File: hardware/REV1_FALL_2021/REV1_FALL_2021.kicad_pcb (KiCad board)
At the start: 2 copper layers, 146 x 133.4 mm, 34 parts, among them J101 Screw_Terminal_01x02, Q101 Q_NMOS_GDS, U1 Teensy3.6_All_Pins, U2 PA16165_Breakout, U201 TPS2113ADRBR, U3 MPL3115A2_Breakout, U301 TPS2113ADRBR, U4 BNO055_Breakout, U5 RFM69HCW_Breakout

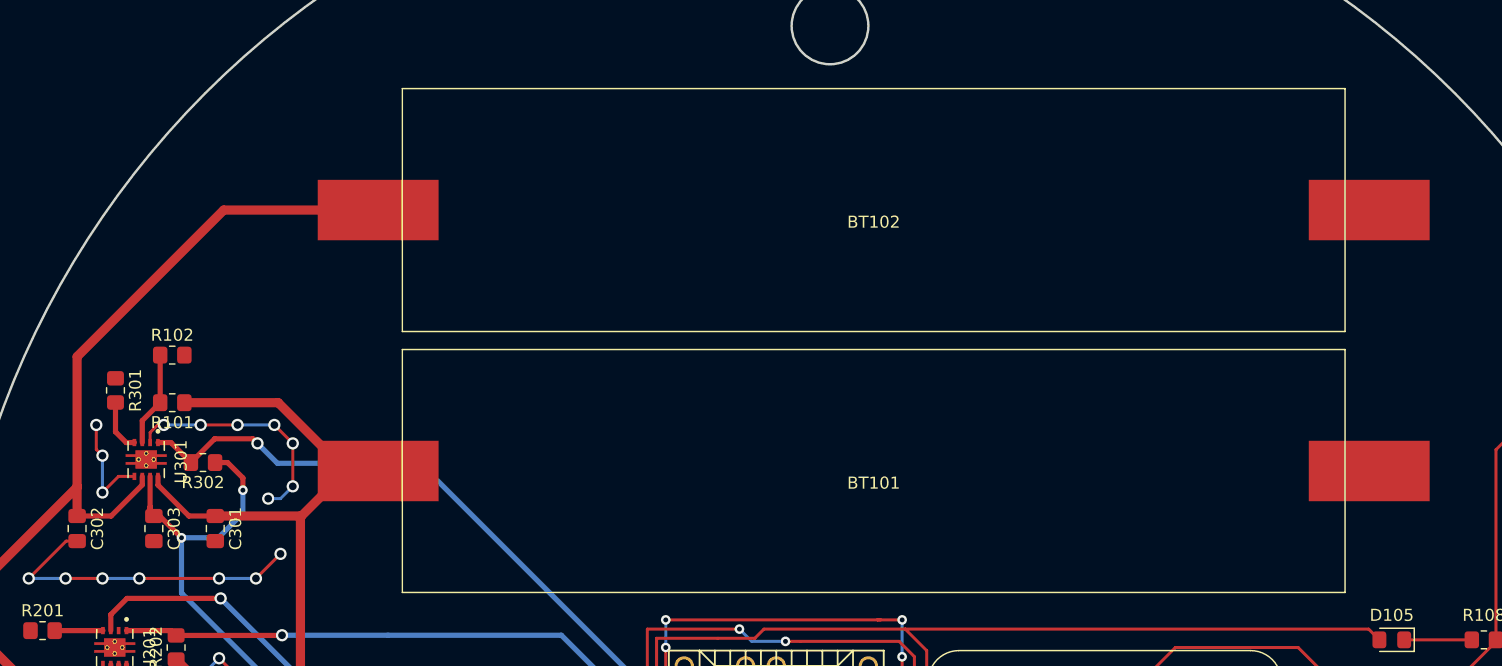
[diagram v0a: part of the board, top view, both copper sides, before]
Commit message: tweak battery positions
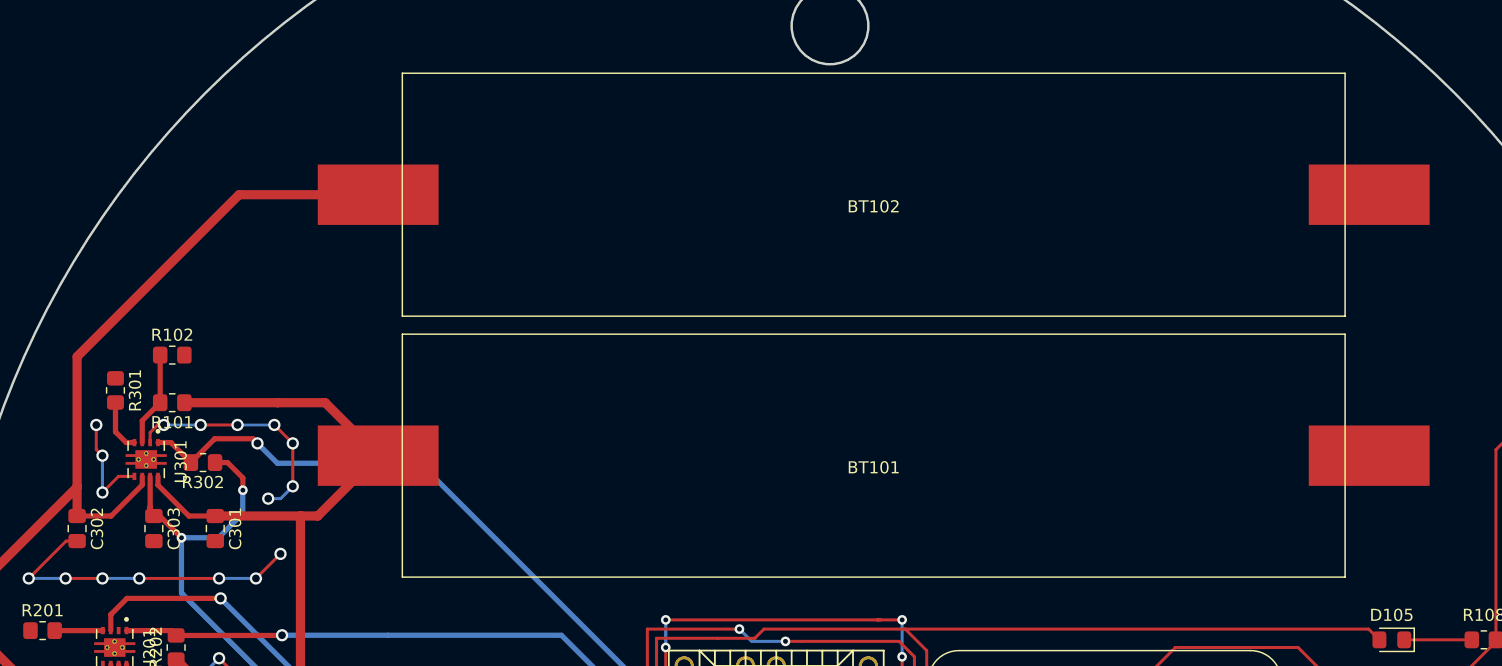
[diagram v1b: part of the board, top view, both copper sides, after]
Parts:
- moved BT102 1.27 mm to (67.9, 59.7)
- moved BT101 1.27 mm to (67.9, 81.3)
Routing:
- net /TPS2113A for E-match/IN2: track 80.9 -> 82.7 mm
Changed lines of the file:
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@@
     (thickness 1.6)
     (drawings 5)
-    (tracks 416)
+    (tracks 417)
     (zones 0)
     (modules 34)
@@
   )
   (setup
-    (last_trace_width 0.25)
+    (last_trace_width 0.762)
     (user_trace_width 0.4318)
     (user_trace_width 0.762)
@@
   )
   (module Olin_Rocketry:MyBatteryHolder_MPD_BH-18650-PC2 (layer F.Cu)
-    (at 67.945 82.55)
+    (at 67.945 81.28)
     (descr "18650 Battery Holder (http://www.memoryprotectiondevices.com/datasheets/BK-18650-PC2-datasheet.pdf)")
     (tags "18650 Battery Holder")
@@
   )
   (module Olin_Rocketry:MyBatteryHolder_MPD_BH-18650-PC2 (layer F.Cu)
-    (at 67.945 60.96)
+    (at 67.945 59.69)
     (descr "18650 Battery Holder (http://www.memoryprotectiondevices.com/datasheets/BK-18650-PC2-datasheet.pdf)")
     (tags "18650 Battery Holder")
@@
   (segment (start 44.9365 102.4675) (end 46.863 102.4675) (width 0.4318) (layer F.Cu) (net 109) (status 800000))
   (segment (start 42.123 99.654) (end 44.9365 102.4675) (width 0.4318) (layer F.Cu) (net 109))
-  (segment (start 62.945 82.55) (end 60.325 82.55) (width 0.762) (layer F.Cu) (net 109) (status C00000))
-  (segment (start 60.325 82.55) (end 56.6 86.275) (width 0.762) (layer F.Cu) (net 109) (status 400000))
   (segment (start 56.6 86.275) (end 56.515 86.275) (width 0.762) (layer F.Cu) (net 109))
   (segment (start 56.515 86.275) (end 49.4665 86.275) (width 0.762) (layer F.Cu) (net 109) (status 800000))
@@
   (segment (start 56.515 99.06) (end 56.515 86.275) (width 0.762) (layer F.Cu) (net 109))
   (segment (start 53.1075 102.4675) (end 56.515 99.06) (width 0.762) (layer F.Cu) (net 109))
-  (segment (start 62.945 82.55) (end 60.325 82.55) (width 0.762) (layer F.Cu) (net 109) (status C00000))
-  (segment (start 60.325 82.55) (end 54.6735 76.8985) (width 0.762) (layer F.Cu) (net 109) (status 400000))
-  (segment (start 54.6735 76.8985) (end 46.9105 76.8985) (width 0.762) (layer F.Cu) (net 109) (status 800000))
+  (segment (start 54.6735 76.8985) (end 54.61 76.8985) (width 0.762) (layer F.Cu) (net 109))
+  (segment (start 54.61 76.8985) (end 46.9105 76.8985) (width 0.762) (layer F.Cu) (net 109) (status 800000))
+  (segment (start 54.61 76.8985) (end 58.5635 76.8985) (width 0.762) (layer F.Cu) (net 109))
+  (segment (start 58.5635 76.8985) (end 62.945 81.28) (width 0.762) (layer F.Cu) (net 109) (status 800000))
+  (segment (start 56.515 86.275) (end 57.95 86.275) (width 0.762) (layer F.Cu) (net 109))
+  (segment (start 57.95 86.275) (end 62.945 81.28) (width 0.762) (layer F.Cu) (net 109) (status 800000))
   (segment (start 43.4265 82.9975) (end 43.4265 83.7005) (width 0.4318) (layer F.Cu) (net 110) (status 400000))
   (segment (start 40.852 86.275) (end 38.0365 86.275) (width 0.4318) (layer F.Cu) (net 110) (status 800000))
@@
   (segment (start 37.9945 102.4675) (end 36.068 102.4675) (width 0.4318) (layer F.Cu) (net 110) (status 800000))
   (segment (start 40.823 99.639) (end 37.9945 102.4675) (width 0.4318) (layer F.Cu) (net 110))
-  (segment (start 62.945 60.96) (end 50.165 60.96) (width 0.762) (layer F.Cu) (net 110) (status 400000))
+  (segment (start 64.215 59.69) (end 51.435 59.69) (width 0.762) (layer F.Cu) (net 110))
   (segment (start 38.0365 73.0885) (end 38.0365 83.82) (width 0.762) (layer F.Cu) (net 110))
   (segment (start 38.0365 83.82) (end 38.0365 86.275) (width 0.762) (layer F.Cu) (net 110) (status 800000))
-  (segment (start 50.165 60.96) (end 38.0365 73.0885) (width 0.762) (layer F.Cu) (net 110))
+  (segment (start 51.435 59.69) (end 38.0365 73.0885) (width 0.762) (layer F.Cu) (net 110))
   (segment (start 38.0365 83.82) (end 38.0365 83.8835) (width 0.762) (layer F.Cu) (net 110))
   (segment (start 31.115 97.3875) (end 36.2165 102.489) (width 0.762) (layer F.Cu) (net 110) (status 800000))
